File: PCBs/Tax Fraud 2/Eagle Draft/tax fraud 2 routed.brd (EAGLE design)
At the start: 34 x 69.1 mm, 10 parts, among them U1 RFM95W-915S2

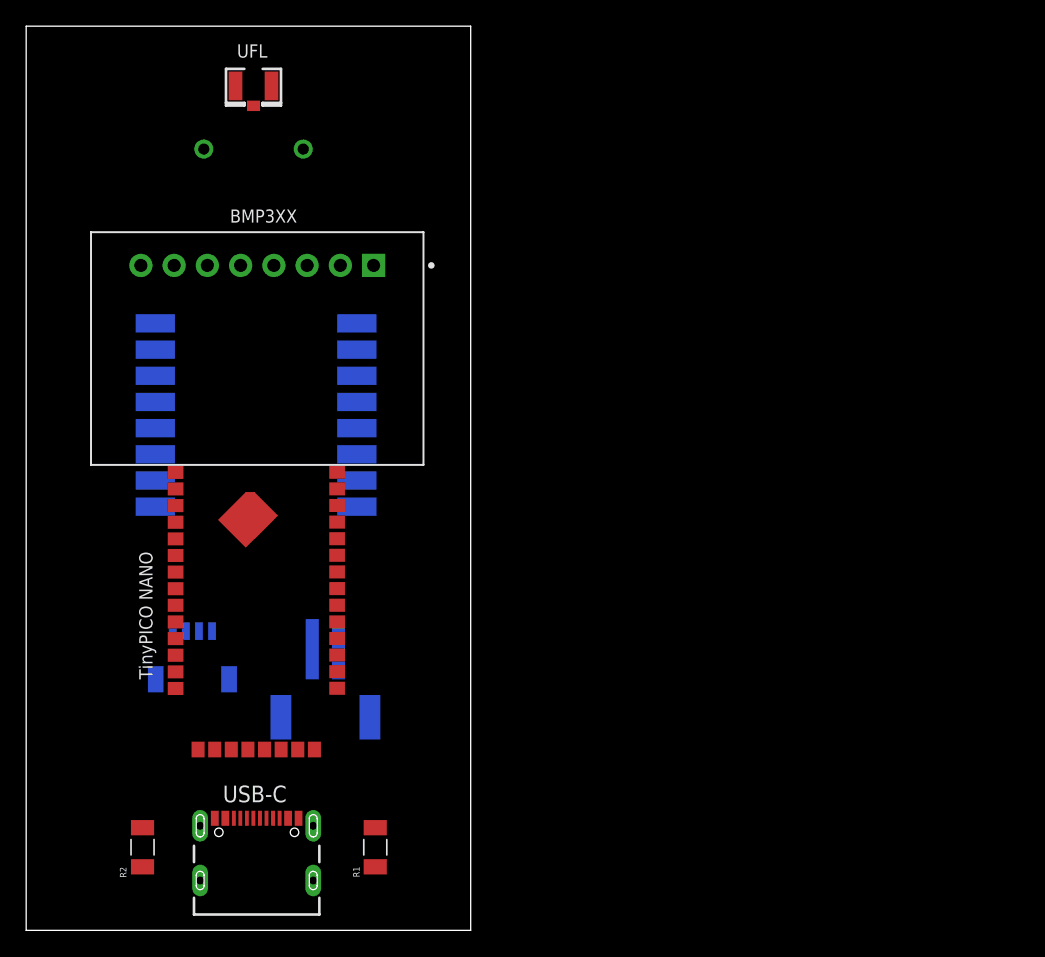
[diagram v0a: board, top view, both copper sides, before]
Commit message: Tax Fraud v2 PCB
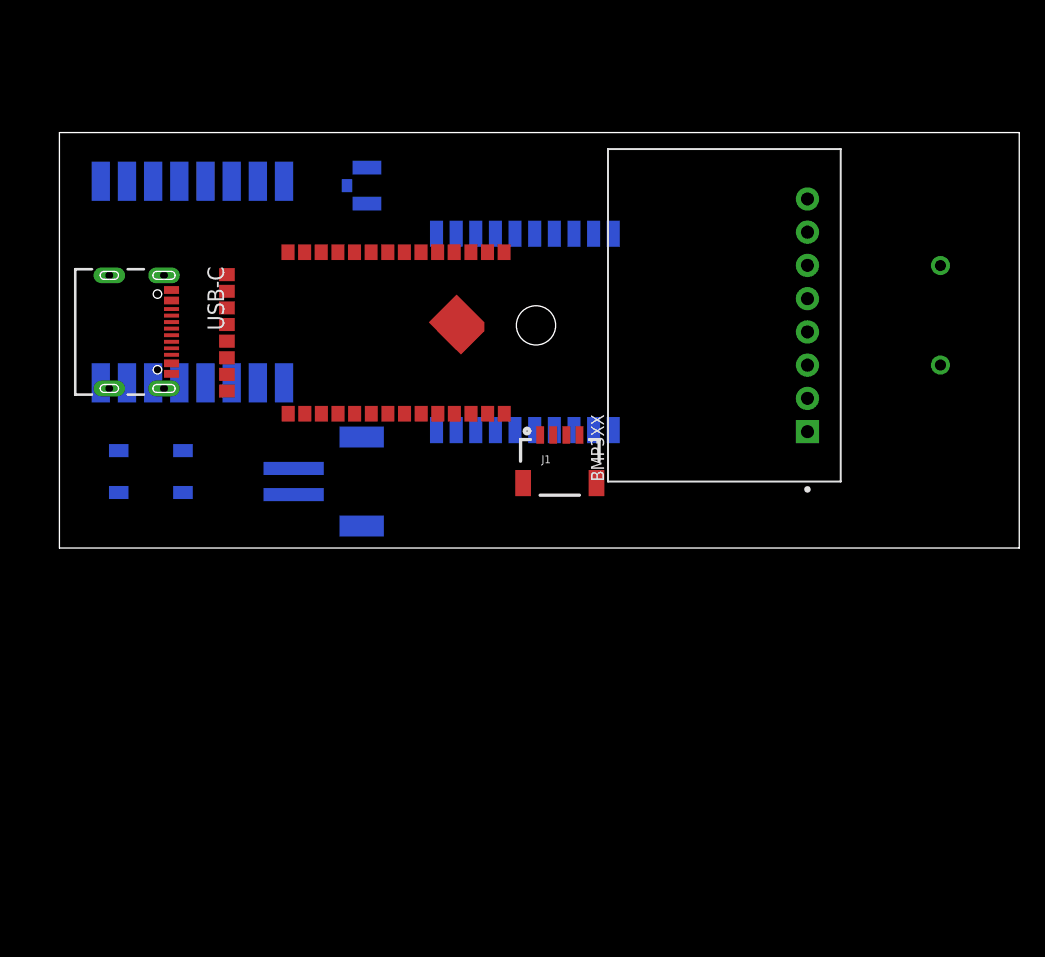
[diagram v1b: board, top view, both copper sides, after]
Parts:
- removed QWIIC: (no value), SparkFun-Connectors:1X04_1MM_RA
- removed R1, R2: CR1206-JW-512ELF, resis CR1206-JW-512ELF:RESC3216X75N
- added D1: 1655, 5050 NeoPixel:LED_1655
- added J1: (no value), SparkFun-Connectors:1X04_1MM_RA
- added U2: (no value), adafruit:FGPMMOPA6H
- moved BEEPER 54.0 mm to (67.3, 47.0), turned to 0 degrees
- moved USB-C 43.4 mm to (3.81, 45.7), turned to 270 degrees
- moved BMP3XX 35.8 mm to (50.8, 47.0), turned to 90 degrees
- moved U$1 27.1 mm to (12.7, 39.4), turned to 0 degrees
- moved JST-PH 16.6 mm to (21.6, 34.3), turned to 90 degrees
- moved UFL 11.5 mm to (23.5, 56.9), flipped to the bottom, turned to 0 degrees
- moved U1 11.3 mm to (10.2, 49.5), turned to 90 degrees
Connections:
- removed net GPIO9: BEEPER.P, U$1.IO9
- removed net N$1: R1.1, USB-C.B5
- removed net N$2: R2.2, USB-C.A5
- removed net N$4: U$1.IO36
- new net BEEP: BEEPER.P, U$1.IO35
- new net FIX: U$1.IO39, U2.P$5
- new net NEO: D1.2, U$1.IO38
- new net RX: U$1.TX, U2.P$10
- new net TX: U$1.RX, U2.P$9
- new net VBACK: U2.P$4
- net GND: now also D1.1, J1.1, U2.P$12, U2.P$19, U2.P$3, U2.P$8; no longer QWIIC.1, R1.2, R2.1
- net SCL: now also J1.4; no longer QWIIC.4
- net SDA: now also J1.3; no longer QWIIC.3
- net VCC: now also J1.2, U2.P$1; no longer QWIIC.2
- net VIN: now also D1.3
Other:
- board size 34 x 69.1 mm -> 73.3 x 31.7 mm
- board text removed: "ANT"
- board text removed: "GND"
- board text removed: "TinyPICO NANO"
